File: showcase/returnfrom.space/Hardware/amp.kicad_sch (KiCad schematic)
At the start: 21 parts, among them U5 LM324

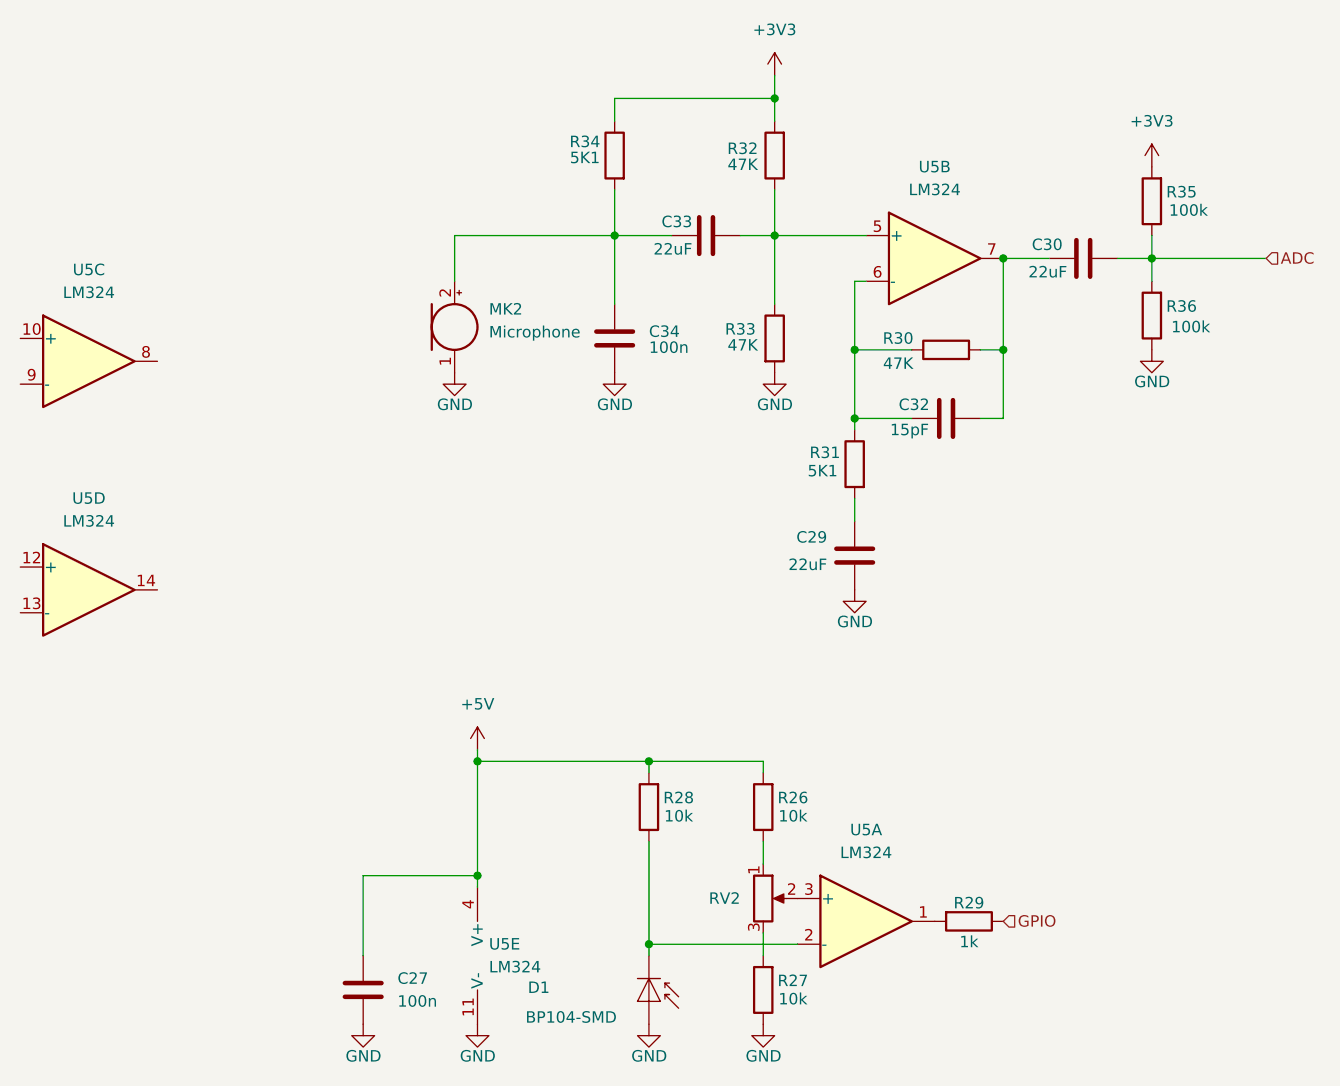
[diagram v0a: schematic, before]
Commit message: panelizing...
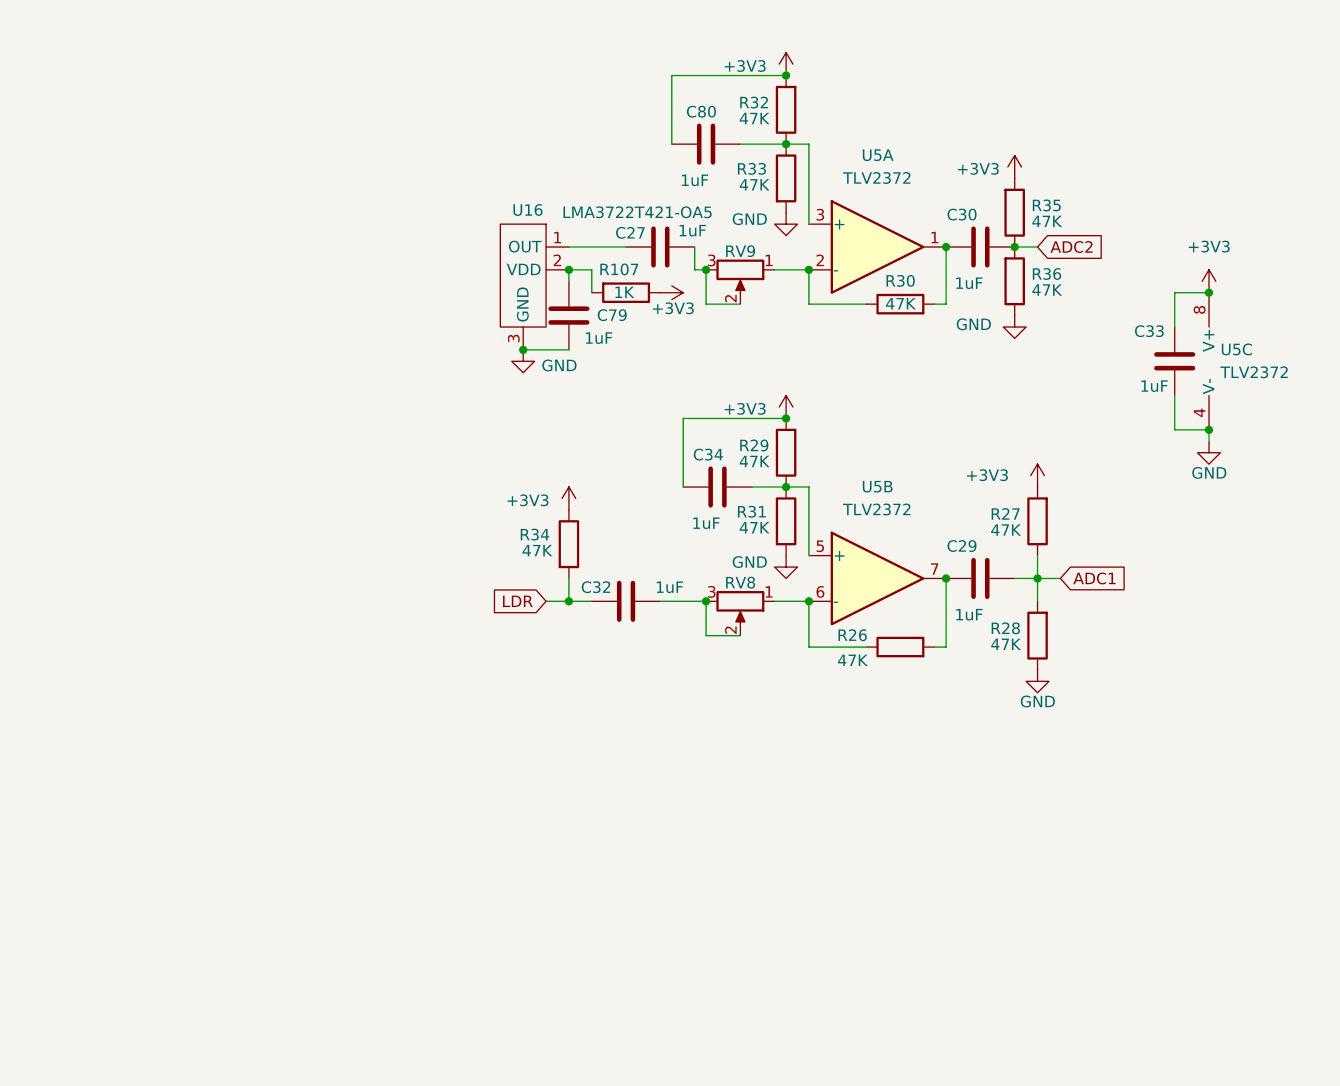
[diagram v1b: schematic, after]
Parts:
- removed D1: BP104-SMD, OptoDevice:Osram_BP104-SMD, symbol Sensor_Optical:BP104-SMD
- removed MK2: Microphone, Sensor_Audio:CUI_CMC-4013-SMT, symbol Device:Microphone
- removed U5: LM324, Package_DIP:DIP-14_W7.62mm_LongPads, symbol Amplifier_Operational:LM324
- added C79, C80: 1uF, Capacitor_SMD:C_0402_1005Metric, symbol Device:C
- added R107: 1K, Resistor_SMD:R_0402_1005Metric, symbol Device:R
- added RV8: R_Potentiometer, Potentiometer_THT:Potentiometer_Runtron_RM-065_Vertical, symbol Device:R_Potentiometer
- added U16: LMA3722T421-OA5, spacescape:LMA3722T421, symbol spacescape:LMA3722T421
- added U5: TLV2372, Package_SO:SOIC-8_3.9x4.9mm_P1.27mm, symbol Amplifier_Operational:TLV2372
- C27, C34: value 100n -> 1uF
- C29, C30, C33: value 22uF -> 1uF; footprint Capacitor_SMD:C_0805_2012Metric -> Capacitor_SMD:C_0402_1005Metric
- C32: value 15pF -> 1uF
- R26, R27, R28: value 10k -> 47K
- R29: value 1k -> 47K
- R31, R34: value 5K1 -> 47K
- R35, R36: value 100k -> 47K
- RV9: renamed from RV2; footprint Potentiometer_SMD:Potentiometer_Bourns_TC33X_Vertical -> Potentiometer_THT:Potentiometer_Runtron_RM-065_Vertical
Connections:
- net +3V3: now also C33.2, C34.1, R27.2, R29.2, C80.1, R107.1, U5.8 (V+)
- net GND: now also C33.1, R28.1, R31.2, C79.1, U16.3 (GND), U16.4 (GND), U5.4 (V-); no longer C27.2, C29.2, C34.2, R27.1
- net at C30.1, R30.2: now also U5.1; no longer C32.2
- net at C29.1: now also R26.2, U5.7; no longer R31.2
- net at R32.1, R33.1: now also C80.2, U5.3 (+); no longer C33.2
- net at R26.1: now also RV8.1, U5.6 (-); no longer RV9.1
- net at RV9.2: now also C27.2, RV9.3
- removed net +5V: C27.1, R26.2, R28.2
- net ADC renamed ADC2
- net GPIO: no longer names the net of R29.1
- net GPIO: now also C34.2, R31.1, U5.5 (+)
- new net: C79.2, R107.2, U16.2 (VDD)
- new net: C27.1, U16.1 (OUT)
- new net: R30.1, RV9.1, U5.2 (-)
- new net: C32.2, RV8.2, RV8.3
- new net ADC1: C29.2, R27.1, R28.2
- new net LDR: C32.1, R34.2
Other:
- moved on the sheet: R30, R32, R33, RV9
